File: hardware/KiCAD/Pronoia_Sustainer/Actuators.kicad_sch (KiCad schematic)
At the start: 33 parts, among them J10 Screw_Terminal_01x02, J3 Screw_Terminal_01x02, J4 Servo0, J5 Servo0, J6 Servo0, J7 Servo0, J8 Screw_Terminal_01x02, J9 Screw_Terminal_01x02, Q1 AO3400A, Q2 AO3400A, Q3 AO3400A, Q4 AO3400A

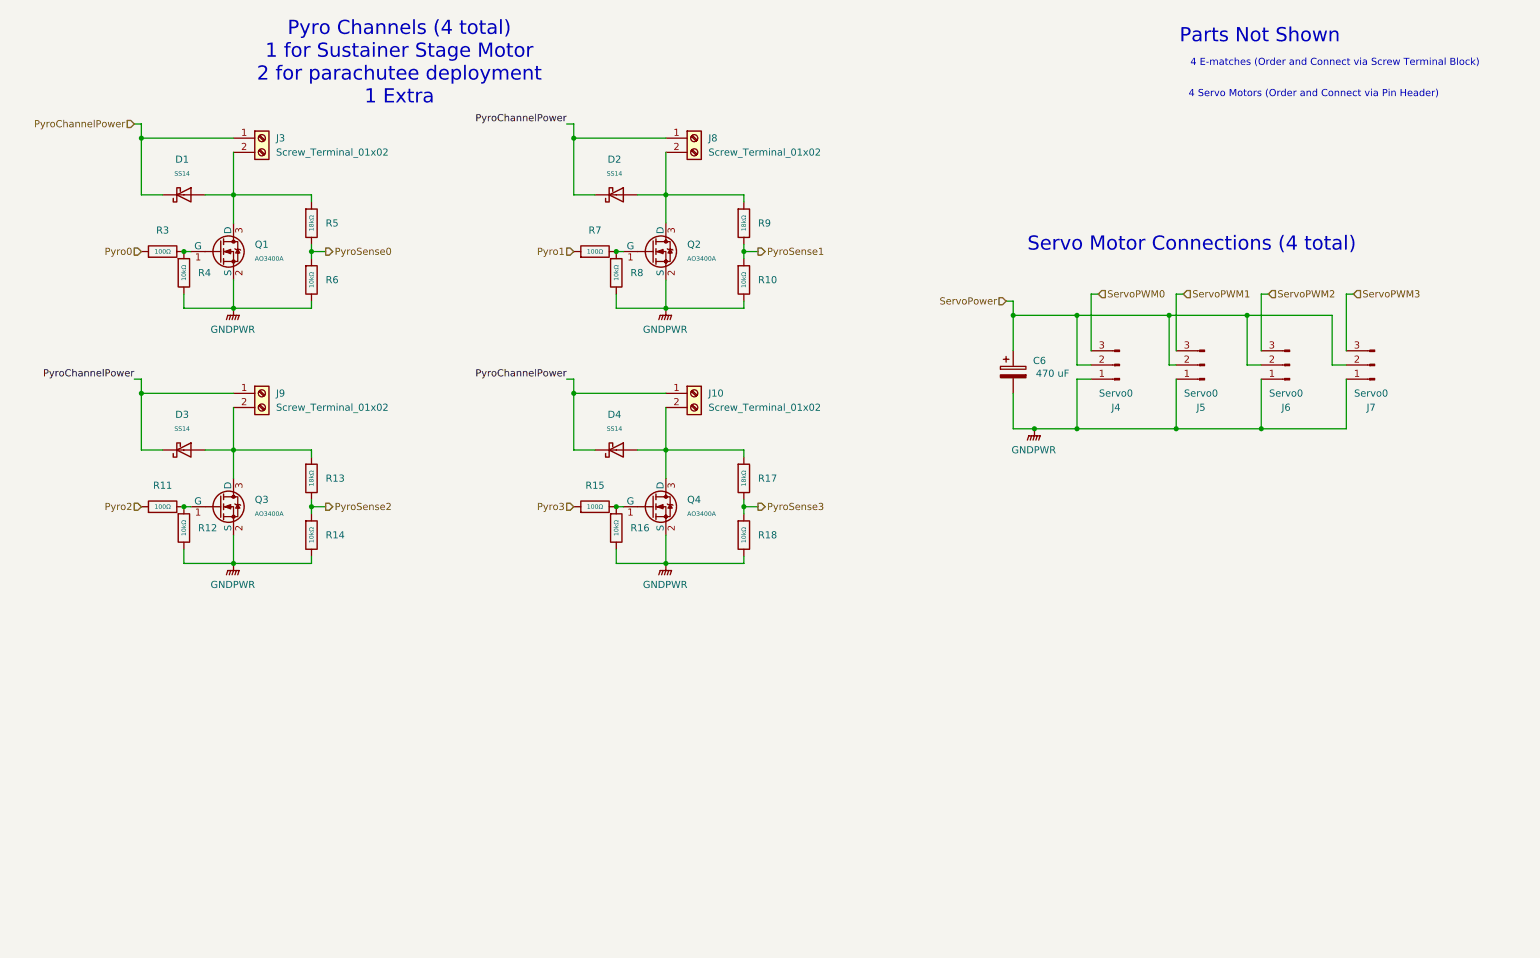
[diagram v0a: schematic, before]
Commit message: Finalized v2.0 of Pronoia Schematic
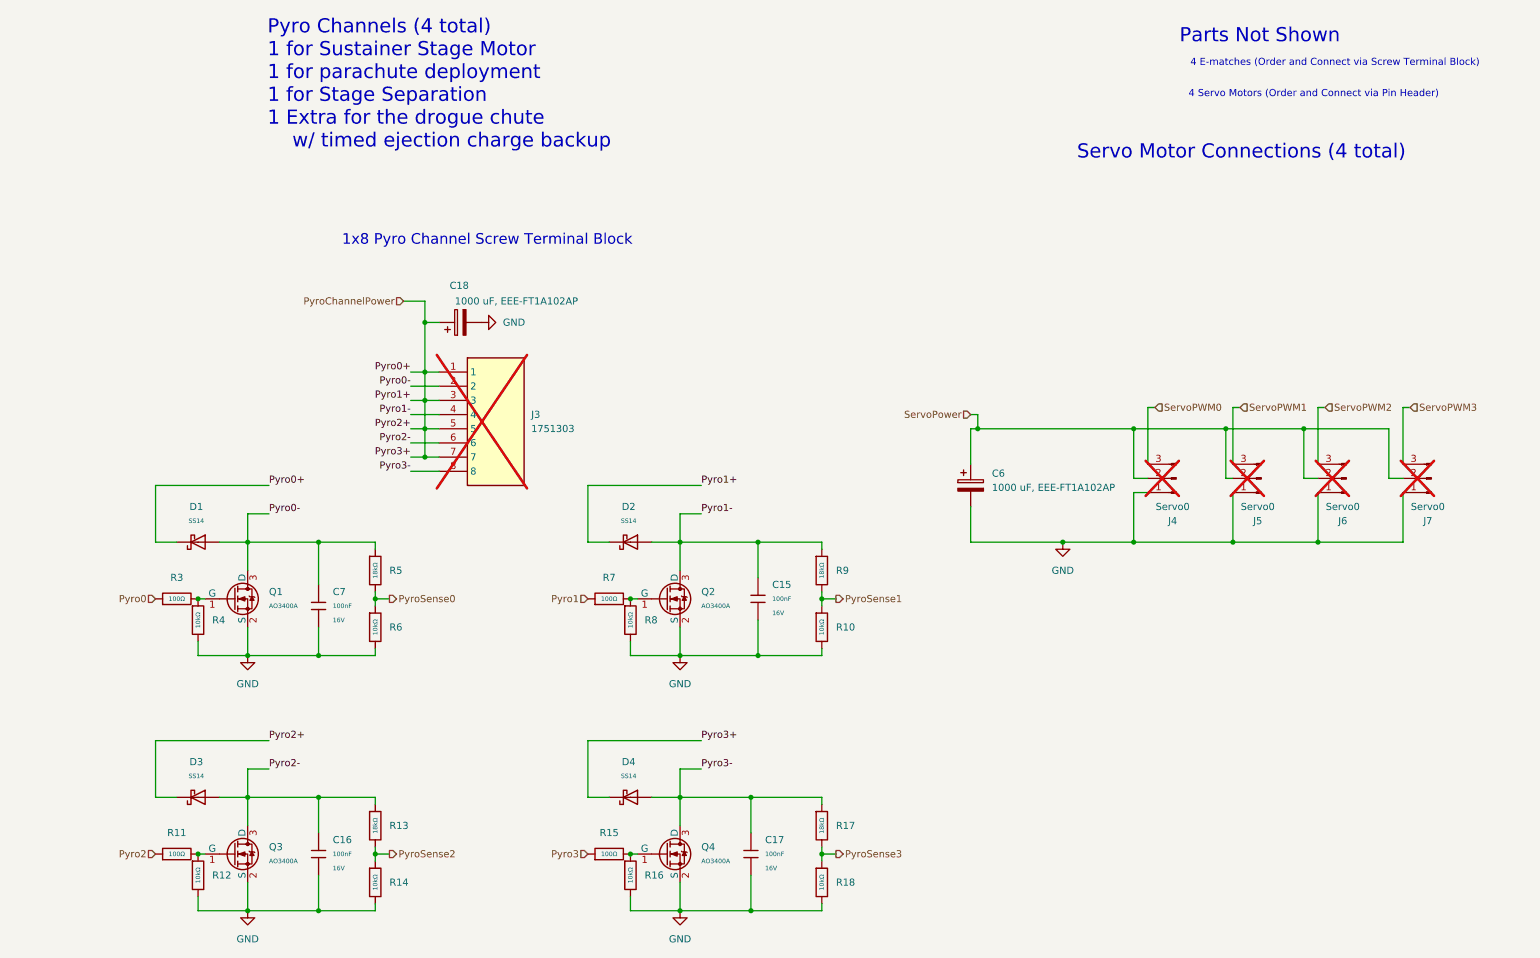
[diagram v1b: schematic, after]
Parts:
- removed J10, J3, J8, J9: Screw_Terminal_01x02, TerminalBlock_Phoenix:TerminalBlock_Phoenix_MKDS-1,5-2-5.08_1x02_P5.08mm_Horizontal, symbol Connector:Screw_Terminal_01x02
- added C15, C16, C17, C7: 100nF, PCM_JLCPCB:C_0402, symbol PCM_JLCPCB-Capacitors:0402,100nF
- added C18: 1000 uF, EEE-FT1A102AP, Capacitor_SMD:CP_Elec_8x10.5, symbol Device:C_Polarized
- added J3: 1751303, 1751303:1751303, symbol 1751303:1751303
- C6: value 470 uF -> 1000 uF, EEE-FT1A102AP; footprint Capacitor_SMD:CP_Elec_8x10 -> Capacitor_SMD:CP_Elec_8x10.5; LCSC C970706 -> C278408
- J4, J5, J6, J7: now not fitted
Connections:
- net PyroChannelPower: now also C18.1, J3.1, J3.3, J3.5, J3.7
- net Pyro1-: now reaches D2.2, Q2.3 (D), R9.1
- net Pyro1-: now also C15.1, J3.4
- net Pyro2-: now reaches D3.2, Q3.3 (D), R13.1
- net Pyro2-: now also C16.1, J3.6
- net Pyro3-: now reaches D4.2, Q4.3 (D), R17.1
- net Pyro3-: now also C17.1, J3.8
- net Pyro0-: now reaches D1.2, Q1.3 (D), R5.1
- net Pyro0-: now also C7.1, J3.2
- net GNDPWR renamed GND
- net GND: now also C15.2, C16.2, C17.2, C18.2, C7.2
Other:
- note added: "1x8 Pyro Channel Screw Terminal Block"
- note added: "Pyro Channels (4 total) 1 for Sustainer Stage Motor 1 for parachute deployment 1 for Stage Separation 1 Extra for the drogue chute w/ timed ejection charge backup"
- note removed: "Pyro Channels (4 total) 1 for Sustainer Stage Motor 2 for parachutee deployment 1 Extra"
- moved on the sheet: D1, D2, D3, D4, Q1, Q2, Q3, Q4, R10, R11, R12, R13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
